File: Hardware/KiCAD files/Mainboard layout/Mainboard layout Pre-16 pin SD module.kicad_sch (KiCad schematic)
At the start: 82 parts, among them J10 Conn_01x02, J11 Conn_01x04, J12 JST_06, J13 Conn_01x08, J14 Conn_01x08, J17 PINHD_1x8_Male, J18 PINHD_1x8_Male, J19 PINHD_1x8_Male, J2 Screw_Terminal_2_P5.00mm, J20 PINHD_1x8_Male, J22 PINHD_1x8_Male, J23 PINHD_1x8_Male, J24 PINHD_1x8_Male, J25 Conn_01x04, J26 Conn_01x04, J27 Conn_01x04, J28 PINHD_1x8_Male, J3 Screw_Terminal_2_P3.50mm, J30 USB-A1VSB6, J31 JST_03, J32 USB-A1VSB6, J34 JST_03, J35 JST_03, J36 JST_03, J37 JST_03, J38 JST_03, J4 JST_06, J5 Conn_01x04, J6 JST_06, J7 JST_06, J8 Conn_01x06, J9 Conn_01x10, Q1 BS170, Q2 2DD1664, SW1 210-4MS, SW2 210-4MS, SW3 210-4MS, SW4 210-4MS, SW8 Push_Button, SW9 Push_Button, U1 CP2102-GM, U12 ESP32-S3-WROOM-1, U2 PCA9534PW_118, U4 PCA9534PW_118

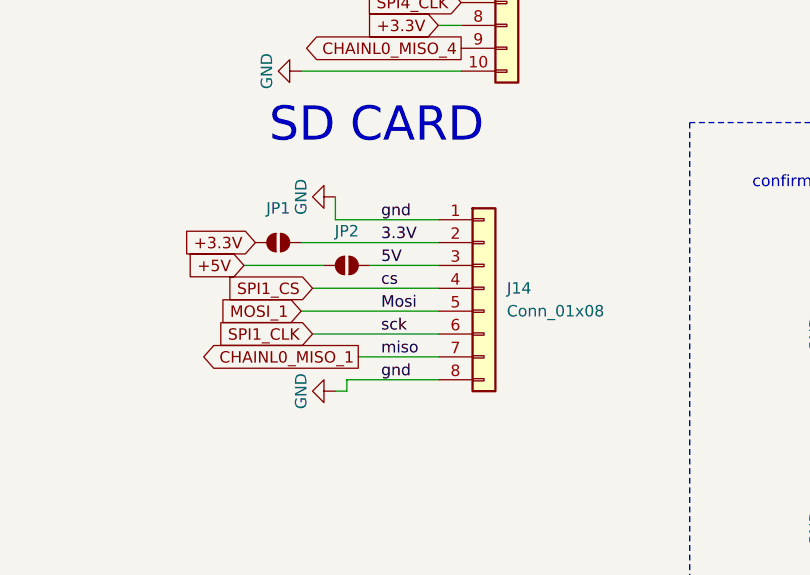
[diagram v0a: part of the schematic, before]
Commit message: Most recent changes to final submission
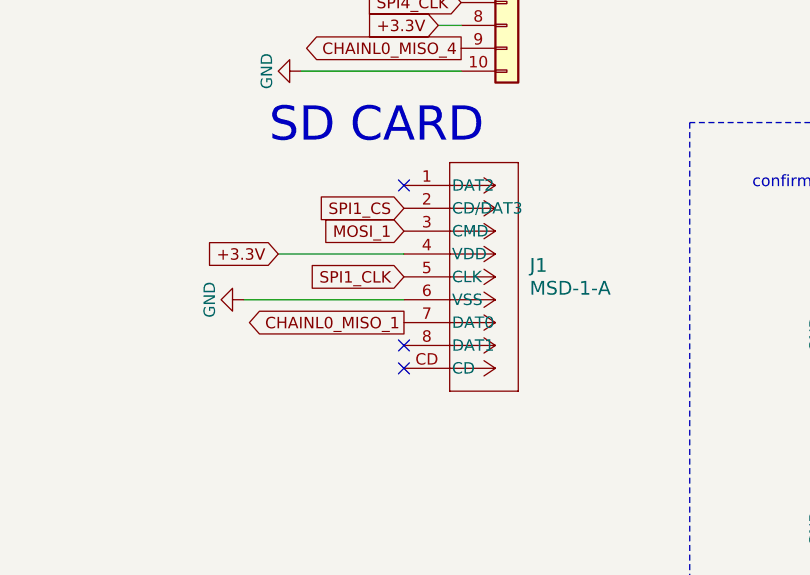
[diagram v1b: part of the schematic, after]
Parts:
- removed J14: Conn_01x08, PCM_SparkFun-Connector:1x08_P2.54mm, symbol PCM_SparkFun-Connector:Conn_01x08_P2.54mm
- removed JP1, JP2: (no value), PCM_SparkFun-Jumper:Jumper_2_NO, symbol PCM_SparkFun-Jumper:SolderJumper_2_Open
- added J1: MSD-1-A, Connector_Card:SD_Hirose_DM1AA_SF_PEJ82, symbol 2026-04-18_00-57-23:MSD-1-A
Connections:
- net 3.3V: now also J1.4 (VDD)
- net CHAINL0_MISO_1: now also J1.7 (DAT0)
- net GND: now also J1.6 (VSS)
- net MOSI_1: now also J1.3 (CMD)
- net SPI1_CLK: now also J1.5 (CLK)
- net SPI1_CS: now also J1.2 (CD/DAT3)
- no-connect marks 33 -> 36
